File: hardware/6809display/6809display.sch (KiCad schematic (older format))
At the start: 36 parts, among them J1 Video Out, J2 To Computer, Q1 BC557, Q2 BC557, Q3 BC557, U1 74HC04, U2 74HC04, U3 74HC393, U4 SAA5020, U5 SAA5050, U6 IDT7132, U7 74HC08, Y1 Crystal

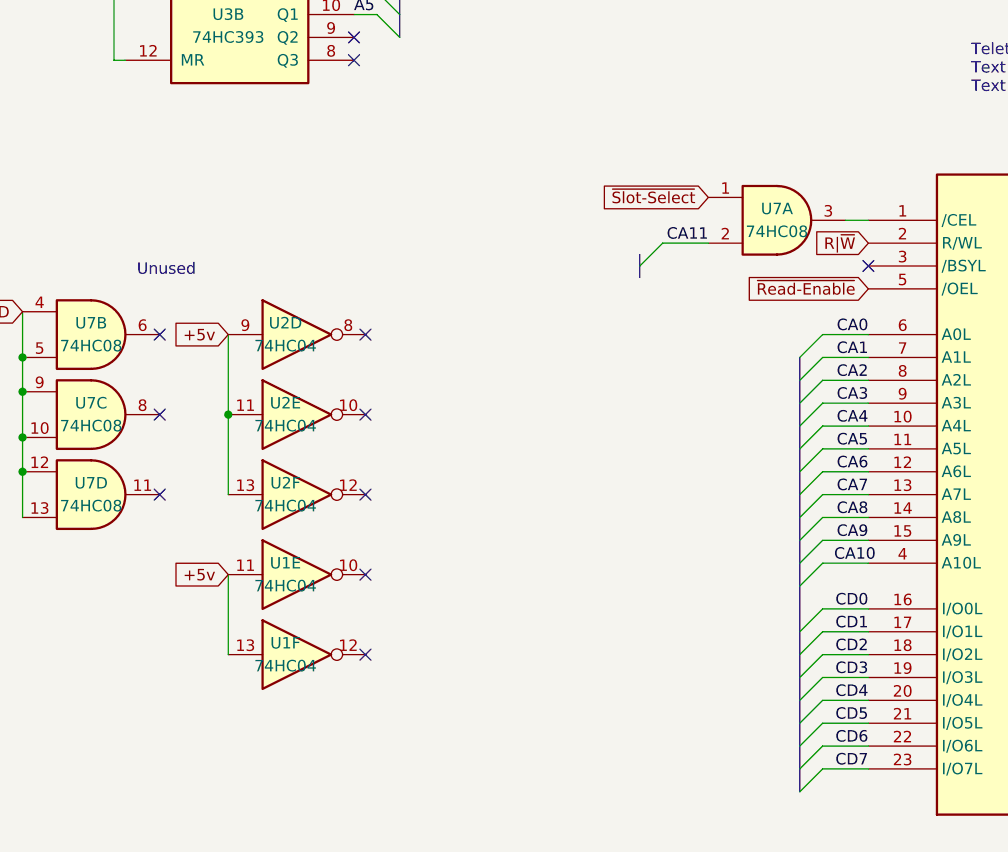
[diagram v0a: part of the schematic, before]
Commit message: ide comtroller
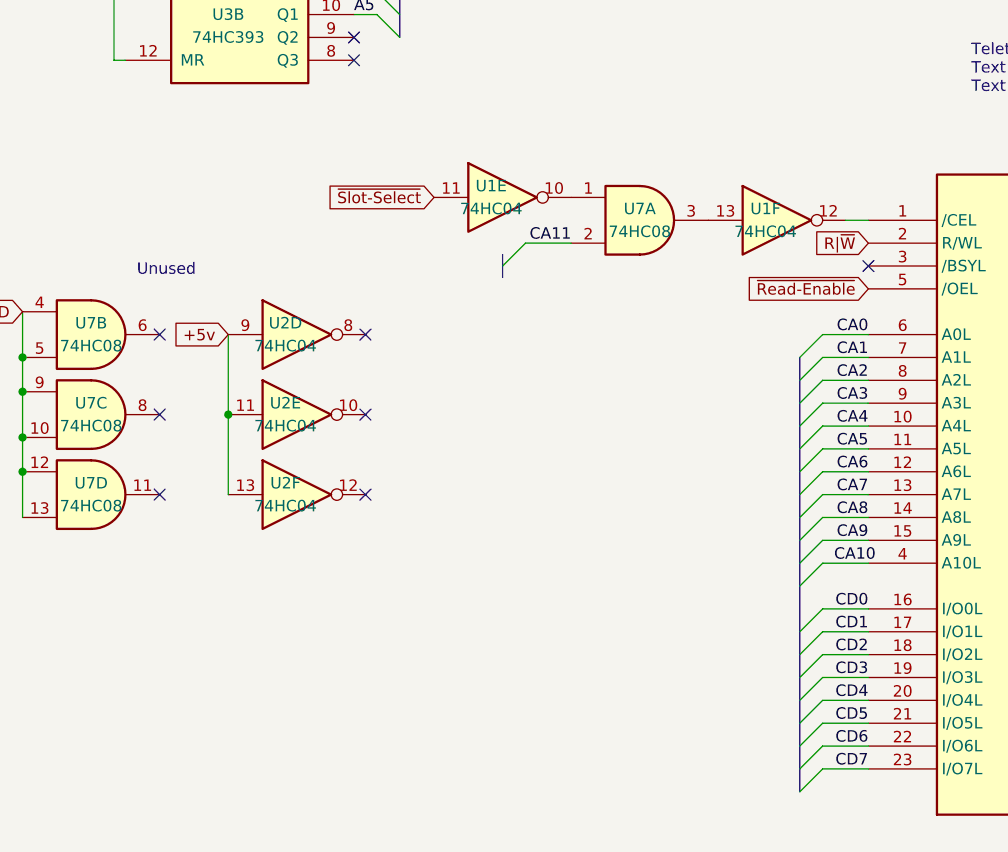
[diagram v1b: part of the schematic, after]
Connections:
- net VCC: no longer U1.11, U1.13
- net ~Slot-Select: now also U1.11; no longer U7.1
- net at U1.10: now also U7.1
- net at U1.12: now also U6.1 (/CEL)
- net at U7.3: now also U1.13; no longer U6.1 (/CEL)
- no-connect marks 40 -> 38
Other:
- moved on the sheet: U1E, U1F, U7A
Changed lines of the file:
@@
 NoConn ~ 5450 6700
 NoConn ~ 5450 7050
-NoConn ~ 5450 7750
-NoConn ~ 5450 7400
 $Comp
 L 74xx:74HC04 U1
 U 6 1 606F7EB3
-P 5150 7750
-F 0 "U1" H 5100 7800 50  0000 C CNN
-F 1 "74HC04" H 5100 7700 50  0000 C CNN
-F 2 "" H 5150 7750 50  0001 C CNN
-F 3 "https://assets.nexperia.com/documents/data-sheet/74HC_HCT04.pdf" H 5150 7750 50  0001 C CNN
-	6    5150 7750
+P 7250 5850
+F 0 "U1" H 7200 5900 50  0000 C CNN
+F 1 "74HC04" H 7200 5800 50  0000 C CNN
+F 2 "" H 7250 5850 50  0001 C CNN
+F 3 "https://assets.nexperia.com/documents/data-sheet/74HC_HCT04.pdf" H 7250 5850 50  0001 C CNN
+	6    7250 5850
 	1    0    0    -1
 $EndComp
@@
 L 74xx:74HC04 U1
 U 5 1 606F65D4
-P 5150 7400
-F 0 "U1" H 5100 7450 50  0000 C CNN
-F 1 "74HC04" H 5100 7350 50  0000 C CNN
-F 2 "" H 5150 7400 50  0001 C CNN
-F 3 "https://assets.nexperia.com/documents/data-sheet/74HC_HCT04.pdf" H 5150 7400 50  0001 C CNN
-	5    5150 7400
+P 6050 5750
+F 0 "U1" H 6000 5800 50  0000 C CNN
+F 1 "74HC04" H 6000 5700 50  0000 C CNN
+F 2 "" H 6050 5750 50  0001 C CNN
+F 3 "https://assets.nexperia.com/documents/data-sheet/74HC_HCT04.pdf" H 6050 5750 50  0001 C CNN
+	5    6050 5750
 	1    0    0    -1
 $EndComp
 Wire Wire Line
 	4850 6700 4850 7050
-Wire Wire Line
-	4850 7400 4850 7750
 Entry Wire Line
 	10750 1400 10850 1500
@@
 Text GLabel 7650 6150 0    50   Input ~ 0
 ~Read-Enable
-Text GLabel 6950 5750 0    50   Input ~ 0
+Text GLabel 5750 5750 0    50   Input ~ 0
 ~Slot-Select
 Entry Wire Line
-	6750 5950 6650 6050
-Text Label 6950 5950 2    50   ~ 0
+	6150 5950 6050 6050
+Text Label 6350 5950 2    50   ~ 0
 CA11
 Wire Wire Line
-	6950 5950 6750 5950
+	6350 5950 6150 5950
 Text Notes 8100 5300 0    50   ~ 0
 Teletext RAM\nText Page 1: E800-EBFF\nText Page 2: EC00-EFFF\n
@@
 L 74xx:74LS08 U7
 U 1 1 6101C4B8
-P 7250 5850
-F 0 "U7" H 7250 5900 50  0000 C CNN
-F 1 "74HC08" H 7250 5800 50  0000 C CNN
-F 2 "" H 7250 5850 50  0001 C CNN
-F 3 "http://www.ti.com/lit/gpn/sn74LS08" H 7250 5850 50  0001 C CNN
-	1    7250 5850
+P 6650 5850
+F 0 "U7" H 6650 5900 50  0000 C CNN
+F 1 "74HC08" H 6650 5800 50  0000 C CNN
+F 2 "" H 6650 5850 50  0001 C CNN
+F 3 "http://www.ti.com/lit/gpn/sn74LS08" H 6650 5850 50  0001 C CNN
+	1    6650 5850
 	1    0    0    -1
 $EndComp
@@
 	1    0    0    -1
 $EndComp
-Text GLabel 4850 7400 0    50   Input ~ 0
-+5v
 Wire Wire Line
 	7650 8250 7450 8250
@@
 Wire Wire Line
 	8950 4100 9050 4100
+$Comp
+L power:PWR_FLAG #FLG0101
+U 1 1 61A719D1
+P 9050 4100
+F 0 "#FLG0101" H 9050 4175 50  0001 C CNN
+F 1 "PWR_FLAG" H 9050 4273 50  0001 C CNN
+F 2 "" H 9050 4100 50  0001 C CNN
+F 3 "~" H 9050 4100 50  0001 C CNN
+	1    9050 4100
+	1    0    0    -1
+$EndComp
+Connection ~ 9050 4100
+Wire Wire Line
+	9050 4100 9150 4100
 Wire Bus Line
-	6650 6000 6650 6100
+	6050 6000 6050 6100
 Wire Bus Line
 	3600 2750 3600 3150
@@
 Wire Bus Line
 	10850 1500 10850 3500
-$Comp
-L power:PWR_FLAG #FLG0101
-U 1 1 61A719D1
-P 9050 4100
-F 0 "#FLG0101" H 9050 4175 50  0001 C CNN
-F 1 "PWR_FLAG" H 9050 4273 50  0001 C CNN
-F 2 "" H 9050 4100 50  0001 C CNN
-F 3 "~" H 9050 4100 50  0001 C CNN
-	1    9050 4100
-	1    0    0    -1
-$EndComp
-Connection ~ 9050 4100
-Wire Wire Line
-	9050 4100 9150 4100
 $EndSCHEMATC

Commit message: text card
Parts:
- added C10, C7, C8, C9: 0.1uF, Capacitor_THT:C_Disc_D5.0mm_W2.5mm_P5.00mm, symbol Device:C
- added NT1: Net-Tie_2, NetTie:NetTie-2_SMD_Pad0.5mm, symbol Device:Net-Tie_2
- added U10, U8, U9: 74HC283, Package_DIP:DIP-16_W7.62mm_LongPads, symbol 74xx:74LS283
- C1, C2, C3, C4, C5, C6: footprint (none) -> Capacitor_THT:C_Disc_D5.0mm_W2.5mm_P5.00mm
- J1: footprint (none) -> Connector_PinHeader_2.54mm:PinHeader_1x05_P2.54mm_Vertical
- J2: footprint SS-50_SS-50_BOARD_CONNECTOR -> Connector_PinHeader_2.54mm:PinHeader_2x25_P2.54mm_Vertical
- R1, R10, R11, R12, R13, R14, R15, R16, R17, R2, R3, R4, R5, R6, R7, R8, R9: footprint (none) -> Resistor_THT:R_Axial_DIN0309_L9.0mm_D3.2mm_P12.70mm_Horizontal
- U1, U2, U3, U7: footprint (none) -> Package_DIP:DIP-14_W7.62mm_LongPads
- U4: footprint (none) -> Package_DIP:DIP-24_W15.24mm_LongPads
- U5: footprint (none) -> Package_DIP:DIP-28_W15.24mm_LongPads
- U6: footprint (none) -> Package_DIP:DIP-48_W15.24mm_LongPads
- Y1: value Crystal -> 6MHz; footprint (none) -> Crystal:Resonator-2Pin_W7.0mm_H2.5mm
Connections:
- net A3: now also U10.1 (S2); no longer U3.13 (CP), U3.6 (Q3)
- net A4: now also U10.13 (S3); no longer U3.11 (Q0)
- net A5: now also U10.10 (S4); no longer U3.10 (Q1)
- net A6: now also U9.4 (S1); no longer U4.19 (A0)
- net A7: now also U9.1 (S2); no longer U4.20 (A1)
- net A8: now also U9.13 (S3); no longer U4.21 (A2)
- net A9: now also U9.10 (S4); no longer U4.22 (A3)
- net GND: now also C1.1, C2.1, C3.1, C5.1, U6.44 (A10R), C10.1, C7.1, C8.1, C9.1, NT1.1, U10.5 (A1), U10.8 (GND), U8.12 (A4), U8.7 (C0), U8.8 (GND), U9.12 (A4), U9.14 (A3), U9.3 (A2), U9.5 (A1), U9.8 (GND); no longer C1.2, C2.2, C3.2, C5.2, U5.2 (~SI)
- net VCC: now also C1.2, C2.2, C3.2, C5.2, C10.2, C7.2, C8.2, C9.2, U10.16 (VCC), U8.16 (VCC), U9.16 (VCC); no longer C1.1, C2.1, C3.1, C5.1
- net A10 renamed SA4
- net SA4: now also U10.6 (B1), U8.14 (A3); no longer U6.44 (A10R)
- new net: U10.3 (A2), U3.13 (CP), U3.6 (Q3)
- new net: U10.12 (A4), U3.10 (Q1)
- new net: U10.14 (A3), U3.11 (Q0)
- new net: NT1.2, U5.2 (~SI)
- new net: U10.11 (B4), U8.4 (S1)
- new net: U10.4 (S1), U9.11 (B4)
- new net: U10.7 (C0), U8.9 (C4)
- new net: U10.9 (C4), U9.7 (C0)
- new net: U8.1 (S2), U9.6 (B1)
- new net: U8.10 (S4), U9.15 (B3)
- new net: U8.13 (S3), U9.2 (B2)
- new net SA0: U10.2 (B2), U4.19 (A0), U8.6 (B1)
- new net SA1: U10.15 (B3), U4.20 (A1), U8.2 (B2)
- new net SA2: U4.21 (A2), U8.15 (B3), U8.5 (A1)
- new net SA3: U4.22 (A3), U8.11 (B4), U8.3 (A2)
- no-connect marks 38 -> 39
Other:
- moved on the sheet: C1, C2, C3, C4, C5, C6, J2, U1E, U1F, U1G, U2D, U2E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

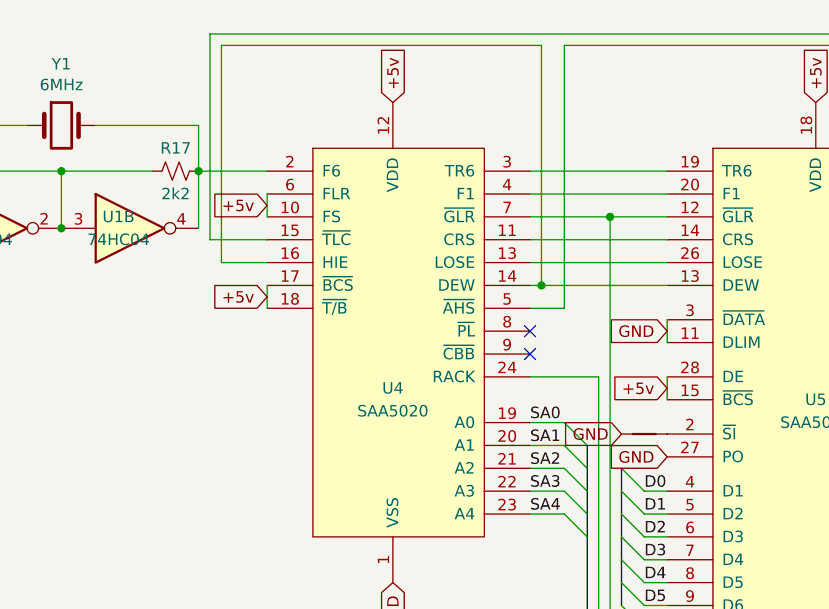
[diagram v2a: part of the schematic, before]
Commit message: clock and more
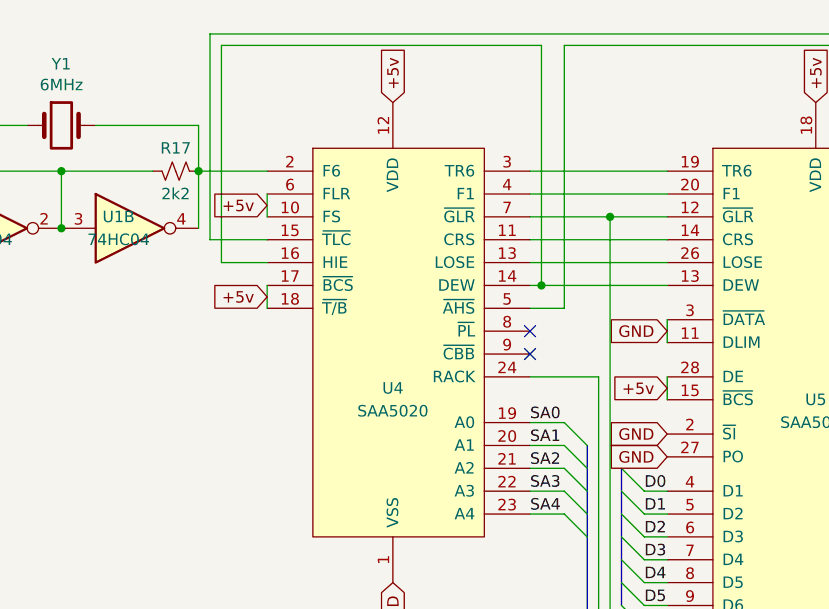
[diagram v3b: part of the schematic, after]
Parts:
- removed NT1: Net-Tie_2, NetTie:NetTie-2_SMD_Pad0.5mm, symbol Device:Net-Tie_2
- R16, R17: footprint Resistor_THT:R_Axial_DIN0309_L9.0mm_D3.2mm_P12.70mm_Horizontal -> Resistor_THT:R_Axial_DIN0207_L6.3mm_D2.5mm_P7.62mm_Horizontal
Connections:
- net GND: now also U5.2 (~SI)
- net at U1.4, U4.2 (F6), Y1.2: now also R17.1; no longer R17.2
- net at R16.2, U1.2, U1.3: now also R17.2; no longer R17.1
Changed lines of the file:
@@
 F 0 "R16" V 900 1550 50  0000 C CNN
 F 1 "2k2" V 700 1550 50  0000 C CNN
-F 2 "Resistor_THT:R_Axial_DIN0309_L9.0mm_D3.2mm_P12.70mm_Horizontal" H 800 1550 50  0001 C CNN
+F 2 "Resistor_THT:R_Axial_DIN0207_L6.3mm_D2.5mm_P7.62mm_Horizontal" H 800 1550 50  0001 C CNN
 F 3 "~" H 800 1550 50  0001 C CNN
 	1    800  1550
@@
 F 0 "R17" V 1900 1550 50  0000 C CNN
 F 1 "2k2" V 1700 1550 50  0000 C CNN
-F 2 "Resistor_THT:R_Axial_DIN0309_L9.0mm_D3.2mm_P12.70mm_Horizontal" H 1800 1550 50  0001 C CNN
+F 2 "Resistor_THT:R_Axial_DIN0207_L6.3mm_D2.5mm_P7.62mm_Horizontal" H 1800 1550 50  0001 C CNN
 F 3 "~" H 1800 1550 50  0001 C CNN
 	1    1800 1550
-	0    -1   -1   0
+	0    1    -1   0
 $EndComp
 Wire Wire Line
@@
 Wire Wire Line
 	3950 2450 3950 2550
-Text GLabel 3750 2700 0    50   Input ~ 0
+Text GLabel 3950 2700 0    50   Input ~ 0
 GND
 Text GLabel 4600 3850 3    50   Input ~ 0
@@
 Text GLabel 3950 2800 0    50   Input ~ 0
 GND
-$Comp
-L Device:Net-Tie_2 NT1
-U 1 1 610191AE
-P 3850 2700
-F 0 "NT1" H 3850 2881 50  0001 C CNN
-F 1 "Net-Tie_2" H 3850 2790 50  0001 C CNN
-F 2 "NetTie:NetTie-2_SMD_Pad0.5mm" H 3850 2700 50  0001 C CNN
-F 3 "~" H 3850 2700 50  0001 C CNN
-	1    3850 2700
-	1    0    0    -1
-$EndComp
 Connection ~ 3250 10550
 Connection ~ 3250 10850
